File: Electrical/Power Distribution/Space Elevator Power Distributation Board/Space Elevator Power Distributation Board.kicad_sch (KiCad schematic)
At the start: 40 parts, among them J1 Screw_Terminal_01x02, J2 Screw_Terminal_01x02, J3 Screw_Terminal_01x02, J4 Screw_Terminal_01x02, J5 Conn_01x02_Pin, J6 Conn_01x02_Pin, Q1 AO4407A, Q10 AO4407A, Q11 AO4407A, Q12 AO4407A, Q2 Q_NMOS_GDS, Q3 AO4407A, Q4 AO4407A, Q5 AO4407A, Q6 AO4407A, Q7 Q_NMOS_GDS, Q8 Q_NMOS_GDS, Q9 Q_NMOS_GDS, U1 TXU0101DBVR, U2 INA219AIDR

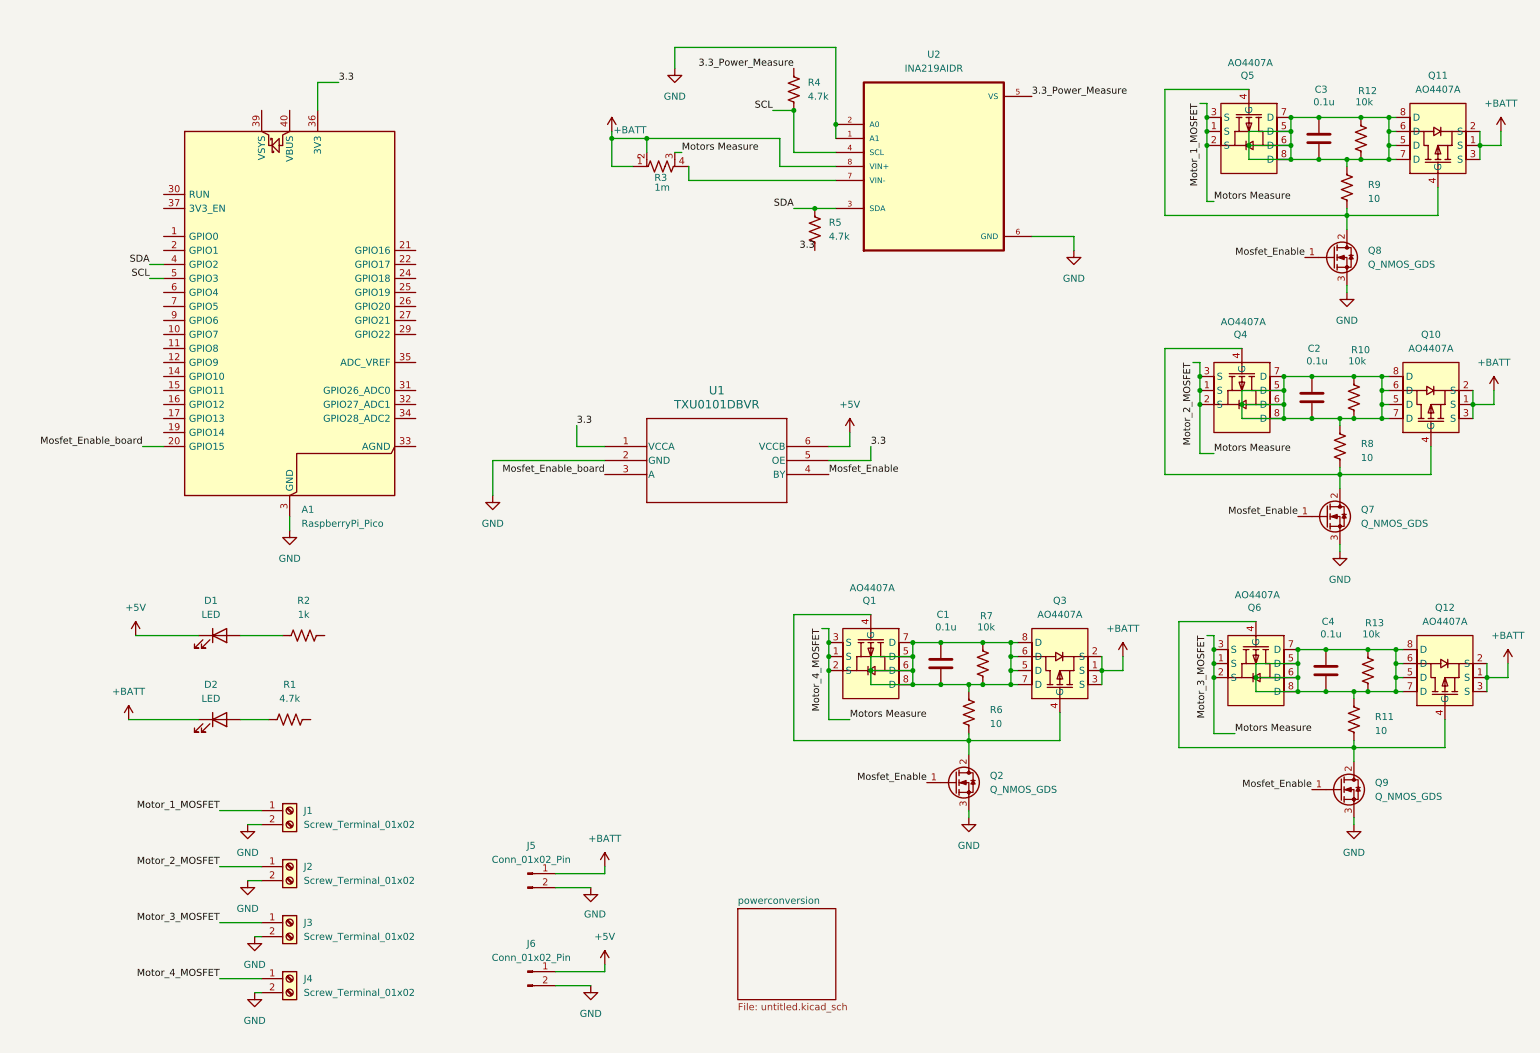
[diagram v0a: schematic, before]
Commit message: Changes to Power Distribution Schematic before PDR
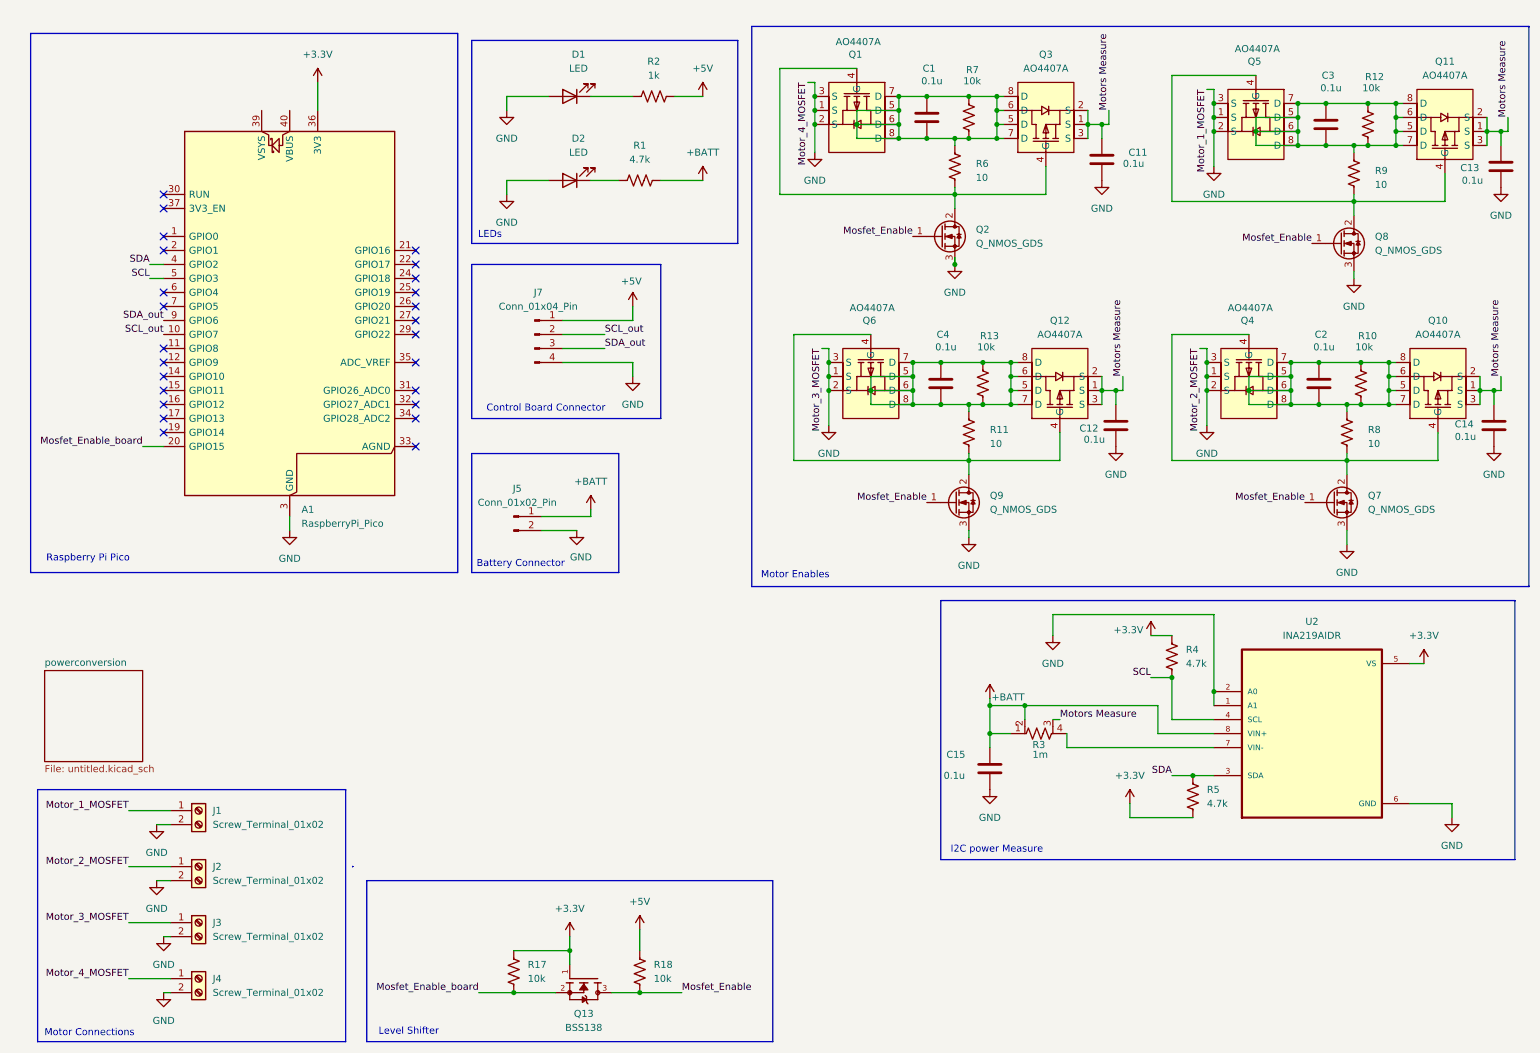
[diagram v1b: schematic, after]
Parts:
- removed J6: Conn_01x02_Pin, symbol Connector:Conn_01x02_Pin
- removed U1: TXU0101DBVR, SOT-23-6-DBV_TEX, symbol 2026-10-16_23-09-01_level_Shifter:TXU0101DBVR
- added C11, C12, C13, C14, C15: 0.1u, symbol Device:C
- added J7: Conn_01x04_Pin, symbol Connector:Conn_01x04_Pin
- added Q13: BSS138, BSS138:SOT95P240X111-3N, symbol BSS138:BSS138
- added R17, R18: 10k, symbol Device:R_US
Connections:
- net 3.3_Power_Measure is gone; now on net +3.3V: R4.1, U2.5 (VS)
- net +5V: now also R2.2, J7.1 (Pin_1), R18.1; no longer D1.1 (K)
- net +BATT: now also R1.2, C15.1; no longer D2.1 (K), Q10.1 (S), Q10.2 (S), Q10.3 (S), Q11.1 (S), Q11.2 (S), Q11.3 (S), Q12.1 (S), Q12.2 (S), Q12.3 (S), Q3.1 (S), Q3.2 (S), Q3.3 (S)
- net GND: now also D1.2 (A), D2.2 (A), J1.1 (Pin_1), J2.1 (Pin_1), J3.1 (Pin_1), J4.1 (Pin_1), Q1.1 (S), Q1.2 (S), Q1.3 (S), Q4.1 (S), Q4.2 (S), Q4.3 (S), Q5.1 (S), Q5.2 (S), Q5.3 (S), Q6.1 (S), Q6.2 (S), Q6.3 (S), C11.2, C12.2, C13.2, C14.2, C15.2, J7.4 (Pin_4)
- net Mosfet_Enable: now also Q13.3, R18.2
- net Mosfet_Enable_board: now also Q13.2, R17.2
- net SCL_out: now reaches A1.10 (GPIO7)
- net SCL_out: now also J7.2 (Pin_2)
- net SDA_out: now reaches A1.9 (GPIO6)
- net SDA_out: now also J7.3 (Pin_3)
- net at R1.1: now also D2.1 (K); no longer D2.2 (A)
- net at R2.1: now also D1.1 (K); no longer D1.2 (A)
- net 3.3 renamed +3.3V
- net +3.3V: now also Q13.1, R17.1
- removed net Motor_1_MOSFET: J1.1 (Pin_1), J2.1 (Pin_1), J3.1 (Pin_1), J4.1 (Pin_1), Q1.1 (S), Q1.2 (S), Q1.3 (S), Q4.1 (S), Q4.2 (S), Q4.3 (S), Q5.1 (S), Q5.2 (S), Q5.3 (S), Q6.1 (S), Q6.2 (S), Q6.3 (S), R3.3
- new net Motors Measure: C11.1, C12.1, C13.1, C14.1, Q10.1 (S), Q10.2 (S), Q10.3 (S), Q11.1 (S), Q11.2 (S), Q11.3 (S), Q12.1 (S), Q12.2 (S), Q12.3 (S), Q3.1 (S), Q3.2 (S), Q3.3 (S), R3.3
- no-connect marks 0 -> 25
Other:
- note added: "Battery Connector"
- note added: "Control Board Connector"
- note added: "I2C power Measure"
- note added: "LEDs"
- note added: "Level Shifter"
- note added: "Motor Connections"
- note added: "Motor Enables"
- note added: "Raspberry Pi Pico"
- moved on the sheet: C1, C2, C3, C4, D1, D2, J1, J2, J3, J4, J5, Q1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
